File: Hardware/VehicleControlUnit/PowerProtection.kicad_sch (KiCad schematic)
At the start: 18 parts, among them IC1 LM74502DDFR, Q1 PSMN012-100YS, Q2 PSMN012-100YS

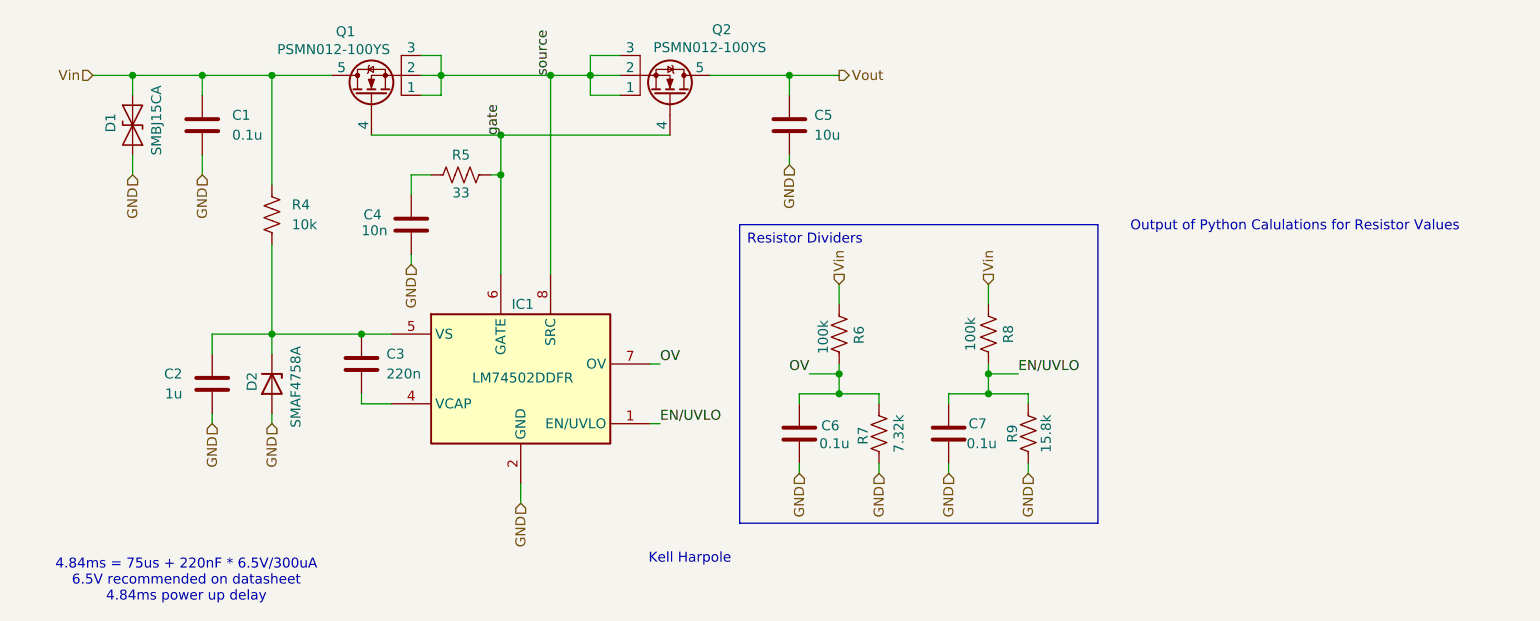
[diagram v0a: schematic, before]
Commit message: 70% tracing done
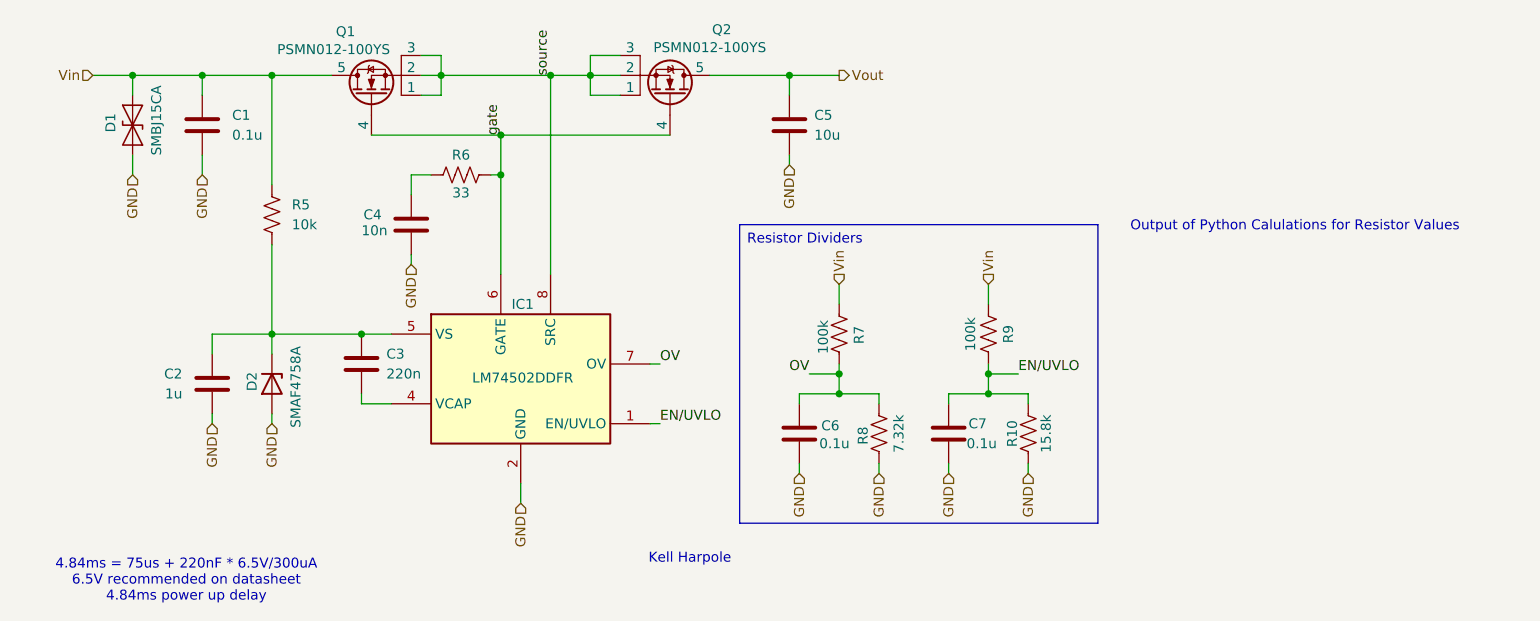
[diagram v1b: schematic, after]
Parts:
- renumbered R9 to R10, R4 to R5, R5 to R6, R6 to R7, R7 to R8, R8 to R9
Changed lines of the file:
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@@
 		(dnp no)
 		(fields_autoplaced yes)
-		(property "Reference" "R4"
+		(property "Reference" "R5"
 			(at 45.72 60.9599 0)
 			(show_name no)
@@
 			(project "VehicleControlUnit"
 				(path "/e864fac9-3897-46c9-9101-6d5488c6cd3a/f16a8bc3-f058-4d27-badd-0afc148d009e/3fe1e163-4ca3-4766-9a9b-19e149cc385e"
-					(reference "R4")
+					(reference "R5")
 					(unit 1)
 				)
@@
 		(in_pos_files yes)
 		(dnp no)
-		(property "Reference" "R9"
+		(property "Reference" "R10"
 			(at 137.668 90.17 90)
 			(show_name no)
@@
 			(project "VehicleControlUnit"
 				(path "/e864fac9-3897-46c9-9101-6d5488c6cd3a/f16a8bc3-f058-4d27-badd-0afc148d009e/3fe1e163-4ca3-4766-9a9b-19e149cc385e"
-					(reference "R9")
+					(reference "R10")
 					(unit 1)
 				)
@@
 		(in_pos_files yes)
 		(dnp no)
-		(property "Reference" "R5"
+		(property "Reference" "R6"
 			(at 67.31 54.61 90)
 			(show_name no)
@@
 			(project "VehicleControlUnit"
 				(path "/e864fac9-3897-46c9-9101-6d5488c6cd3a/f16a8bc3-f058-4d27-badd-0afc148d009e/3fe1e163-4ca3-4766-9a9b-19e149cc385e"
-					(reference "R5")
+					(reference "R6")
 					(unit 1)
 				)
@@
 		(in_pos_files yes)
 		(dnp no)
-		(property "Reference" "R7"
+		(property "Reference" "R8"
 			(at 118.618 90.424 90)
 			(show_name no)
@@
 			(project "VehicleControlUnit"
 				(path "/e864fac9-3897-46c9-9101-6d5488c6cd3a/f16a8bc3-f058-4d27-badd-0afc148d009e/3fe1e163-4ca3-4766-9a9b-19e149cc385e"
-					(reference "R7")
+					(reference "R8")
 					(unit 1)
 				)
@@
 		(in_pos_files yes)
 		(dnp no)
-		(property "Reference" "R6"
+		(property "Reference" "R7"
 			(at 118.11 78.74 90)
 			(show_name no)
@@
 			(project "VehicleControlUnit"
 				(path "/e864fac9-3897-46c9-9101-6d5488c6cd3a/f16a8bc3-f058-4d27-badd-0afc148d009e/3fe1e163-4ca3-4766-9a9b-19e149cc385e"
-					(reference "R6")
+					(reference "R7")
 					(unit 1)
 				)
@@
 		(in_pos_files yes)
 		(dnp no)
-		(property "Reference" "R8"
+		(property "Reference" "R9"
 			(at 137.16 77.47 90)
 			(show_name no)
@@
 			(project "VehicleControlUnit"
 				(path "/e864fac9-3897-46c9-9101-6d5488c6cd3a/f16a8bc3-f058-4d27-badd-0afc148d009e/3fe1e163-4ca3-4766-9a9b-19e149cc385e"
-					(reference "R8")
-					(unit 1)
-				)
+					(reference "R9")
+					(unit 1)
+				)

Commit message: i hate this moco, its so stupid why are we doign this.
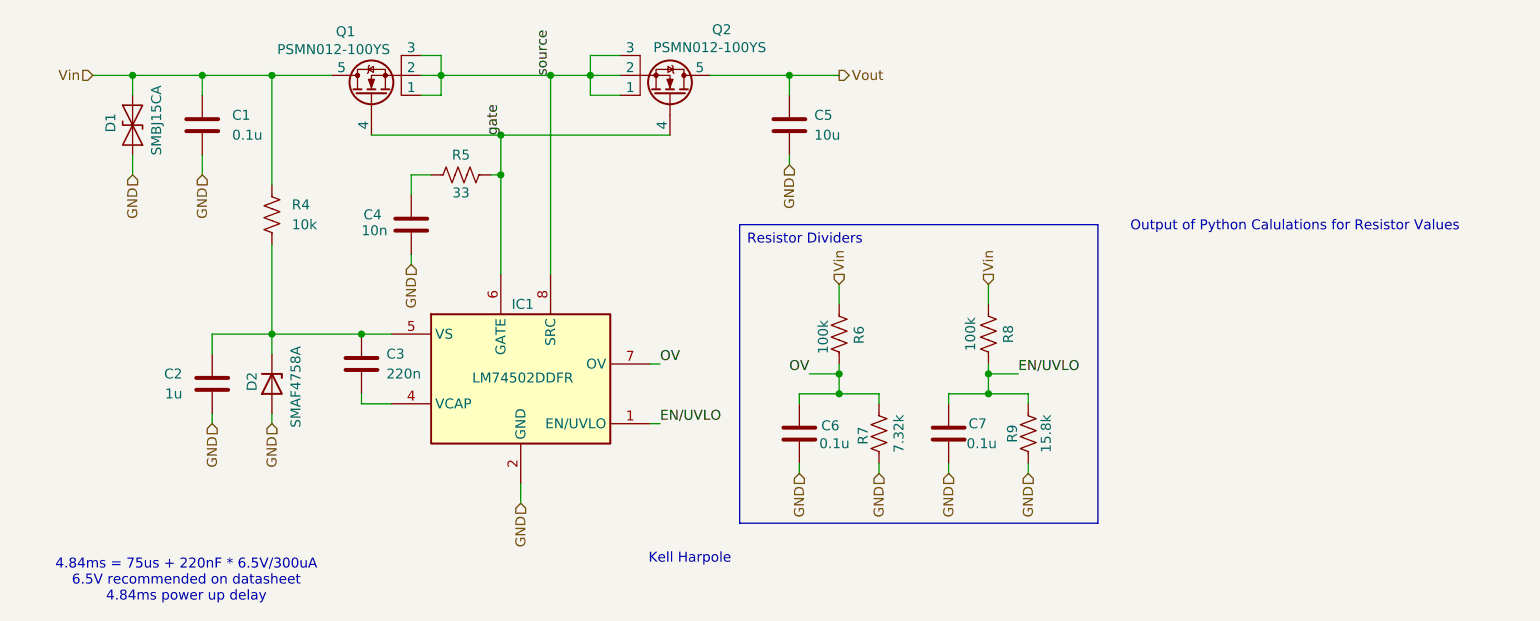
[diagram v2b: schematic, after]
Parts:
- renumbered R5 to R4, R6 to R5, R7 to R6, R8 to R7, R9 to R8, R10 to R9
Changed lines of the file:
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@@
 		(dnp no)
 		(fields_autoplaced yes)
-		(property "Reference" "R5"
+		(property "Reference" "R4"
 			(at 45.72 60.9599 0)
 			(show_name no)
@@
 			(project "VehicleControlUnit"
 				(path "/e864fac9-3897-46c9-9101-6d5488c6cd3a/f16a8bc3-f058-4d27-badd-0afc148d009e/3fe1e163-4ca3-4766-9a9b-19e149cc385e"
-					(reference "R5")
+					(reference "R4")
 					(unit 1)
 				)
@@
 		(in_pos_files yes)
 		(dnp no)
-		(property "Reference" "R10"
+		(property "Reference" "R9"
 			(at 137.668 90.17 90)
 			(show_name no)
@@
 			(project "VehicleControlUnit"
 				(path "/e864fac9-3897-46c9-9101-6d5488c6cd3a/f16a8bc3-f058-4d27-badd-0afc148d009e/3fe1e163-4ca3-4766-9a9b-19e149cc385e"
-					(reference "R10")
+					(reference "R9")
 					(unit 1)
 				)
@@
 		(in_pos_files yes)
 		(dnp no)
-		(property "Reference" "R6"
+		(property "Reference" "R5"
 			(at 67.31 54.61 90)
 			(show_name no)
@@
 			(project "VehicleControlUnit"
 				(path "/e864fac9-3897-46c9-9101-6d5488c6cd3a/f16a8bc3-f058-4d27-badd-0afc148d009e/3fe1e163-4ca3-4766-9a9b-19e149cc385e"
-					(reference "R6")
+					(reference "R5")
 					(unit 1)
 				)
@@
 		(in_pos_files yes)
 		(dnp no)
-		(property "Reference" "R8"
+		(property "Reference" "R7"
 			(at 118.618 90.424 90)
 			(show_name no)
@@
 			(project "VehicleControlUnit"
 				(path "/e864fac9-3897-46c9-9101-6d5488c6cd3a/f16a8bc3-f058-4d27-badd-0afc148d009e/3fe1e163-4ca3-4766-9a9b-19e149cc385e"
-					(reference "R8")
+					(reference "R7")
 					(unit 1)
 				)
@@
 		(in_pos_files yes)
 		(dnp no)
-		(property "Reference" "R7"
+		(property "Reference" "R6"
 			(at 118.11 78.74 90)
 			(show_name no)
@@
 			(project "VehicleControlUnit"
 				(path "/e864fac9-3897-46c9-9101-6d5488c6cd3a/f16a8bc3-f058-4d27-badd-0afc148d009e/3fe1e163-4ca3-4766-9a9b-19e149cc385e"
-					(reference "R7")
+					(reference "R6")
 					(unit 1)
 				)
@@
 		(in_pos_files yes)
 		(dnp no)
-		(property "Reference" "R9"
+		(property "Reference" "R8"
 			(at 137.16 77.47 90)
 			(show_name no)
@@
 			(project "VehicleControlUnit"
 				(path "/e864fac9-3897-46c9-9101-6d5488c6cd3a/f16a8bc3-f058-4d27-badd-0afc148d009e/3fe1e163-4ca3-4766-9a9b-19e149cc385e"
-					(reference "R9")
-					(unit 1)
-				)
+					(reference "R8")
+					(unit 1)
+				)
